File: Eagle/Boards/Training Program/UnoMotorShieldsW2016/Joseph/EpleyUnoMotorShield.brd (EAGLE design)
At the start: 64 x 66 mm, 6 parts, among them J1 ARDUINO_UNO_R3

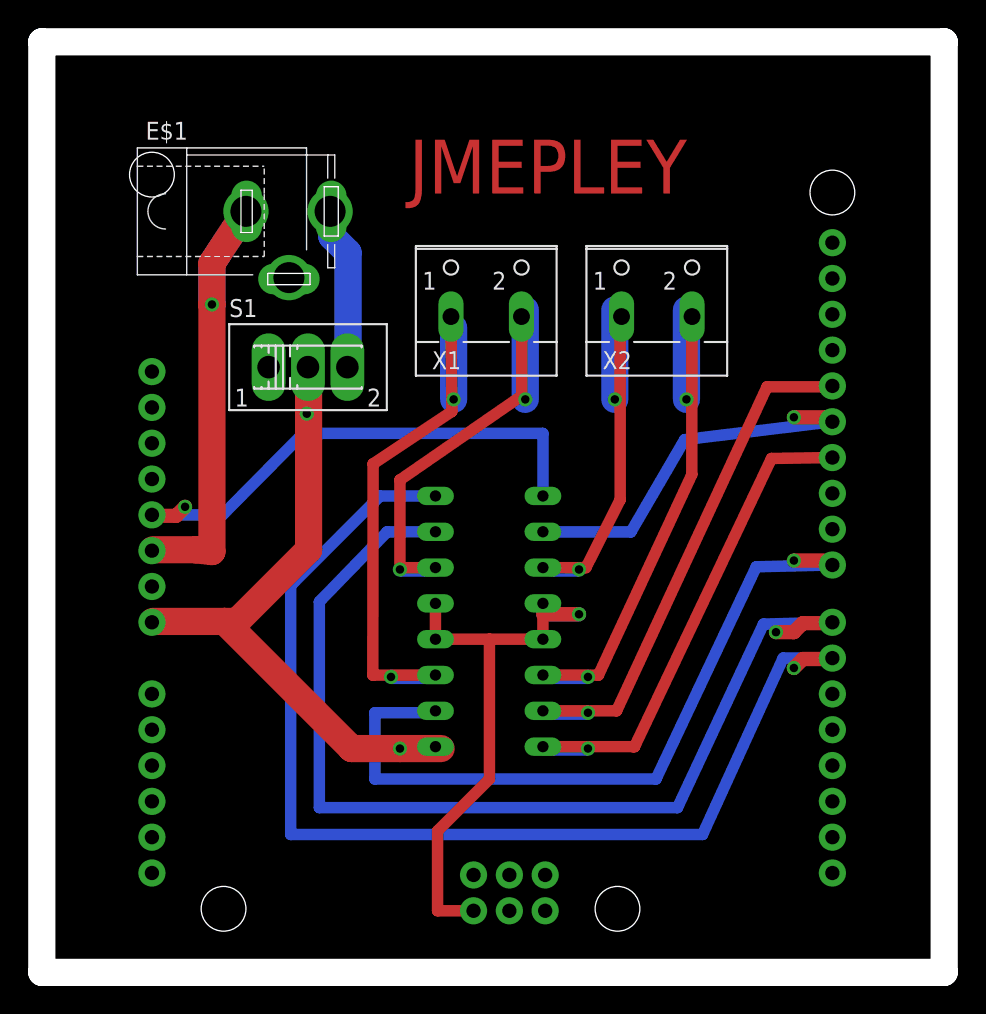
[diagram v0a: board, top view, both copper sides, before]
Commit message: updated Joseph's board
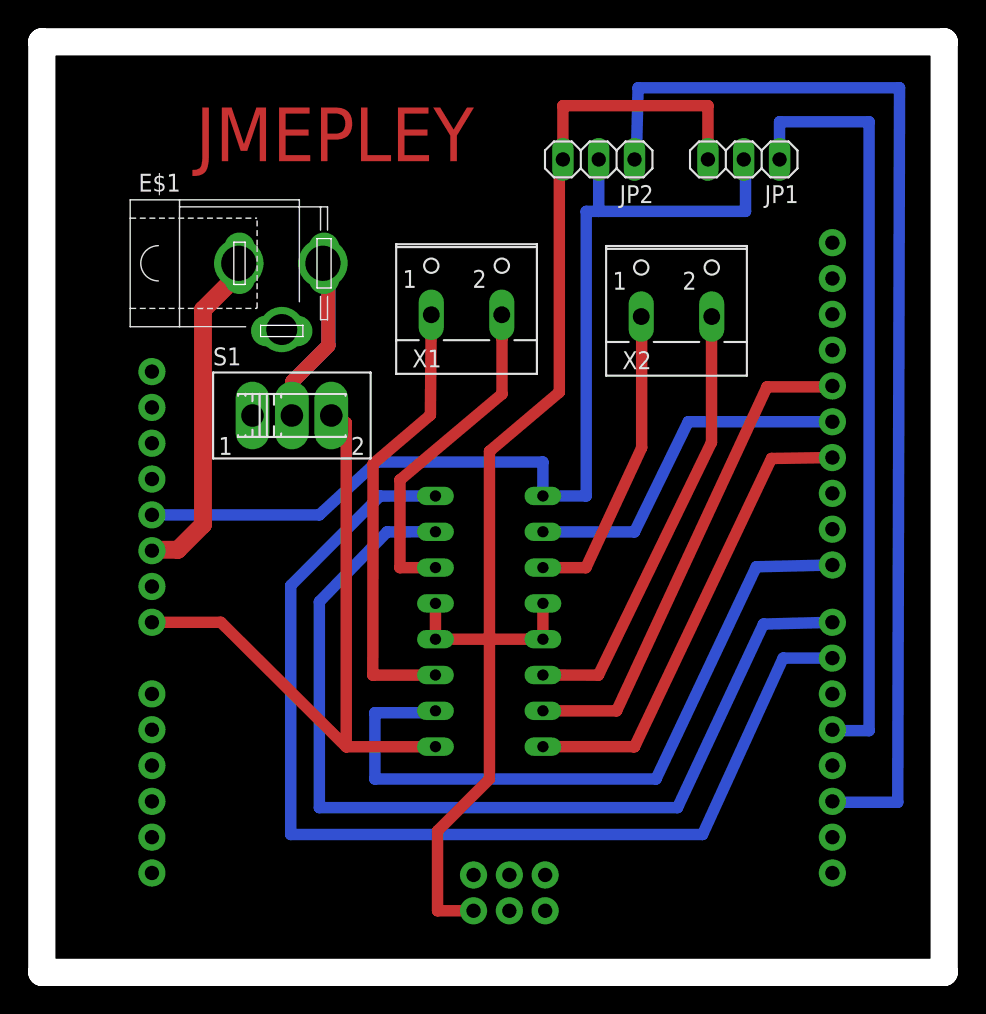
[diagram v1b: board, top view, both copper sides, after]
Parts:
- added JP1, JP2: (no value), ISCTRainingProgram:1X03
- moved E$1 3.72 mm to (17.0, 50.3)
- moved S1 3.61 mm to (17.7, 39.5)
- moved X1 1.40 mm to (30.1, 47.9)
- moved X2 1.40 mm to (45.0, 47.8)
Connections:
- removed net S$1: E$1.P$1
- removed net S$4: S1.3
- new net N$11: J1.D4, JP1.1
- new net N$12: J1.5V, JP1.2, JP2.2, U$1.P16
- net GND: now also JP1.3, JP2.3
- net N$5: now also J1.D2, JP2.1; no longer J1.5V, U$1.P16
- net N$7: now also S1.3
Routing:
- net N$12: track 0.00 -> 73.6 mm
- net N$11: track 0.00 -> 54.9 mm
- net GND: track 36.0 -> 90.4 mm
- net S$5: track 47.7 -> 0.00 mm, vias 1 -> 0
- net N$5: track 34.6 -> 79.1 mm
- net N$7: track 23.8 -> 47.9 mm
- net S$1: track 36.5 -> 23.3 mm, vias 1 -> 0
- net S$3: track 0.00 -> 9.94 mm, vias 1 -> 0
- net S$9: track 6.35 -> 0.00 mm, vias 1 -> 0
- net S$8: track 6.35 -> 0.00 mm, vias 1 -> 0
- net S$7: track 6.35 -> 0.00 mm, vias 1 -> 0
- net S$6: track 5.08 -> 0.00 mm, vias 1 -> 0
- net S$18: track 5.08 -> 0.00 mm, vias 1 -> 0
- net S$21: track 4.07 -> 0.00 mm, vias 1 -> 0
- net S$16: track 3.18 -> 0.00 mm, vias 1 -> 0
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- added copper zone on layer 16, net S$4
- added copper zone on layer 1, net S$5
